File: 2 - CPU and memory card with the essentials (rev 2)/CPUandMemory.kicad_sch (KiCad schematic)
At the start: 9 parts, among them U10 AS6C4008, U7 Z84C0010, U8 SST39SF010, U9 AS6C4008

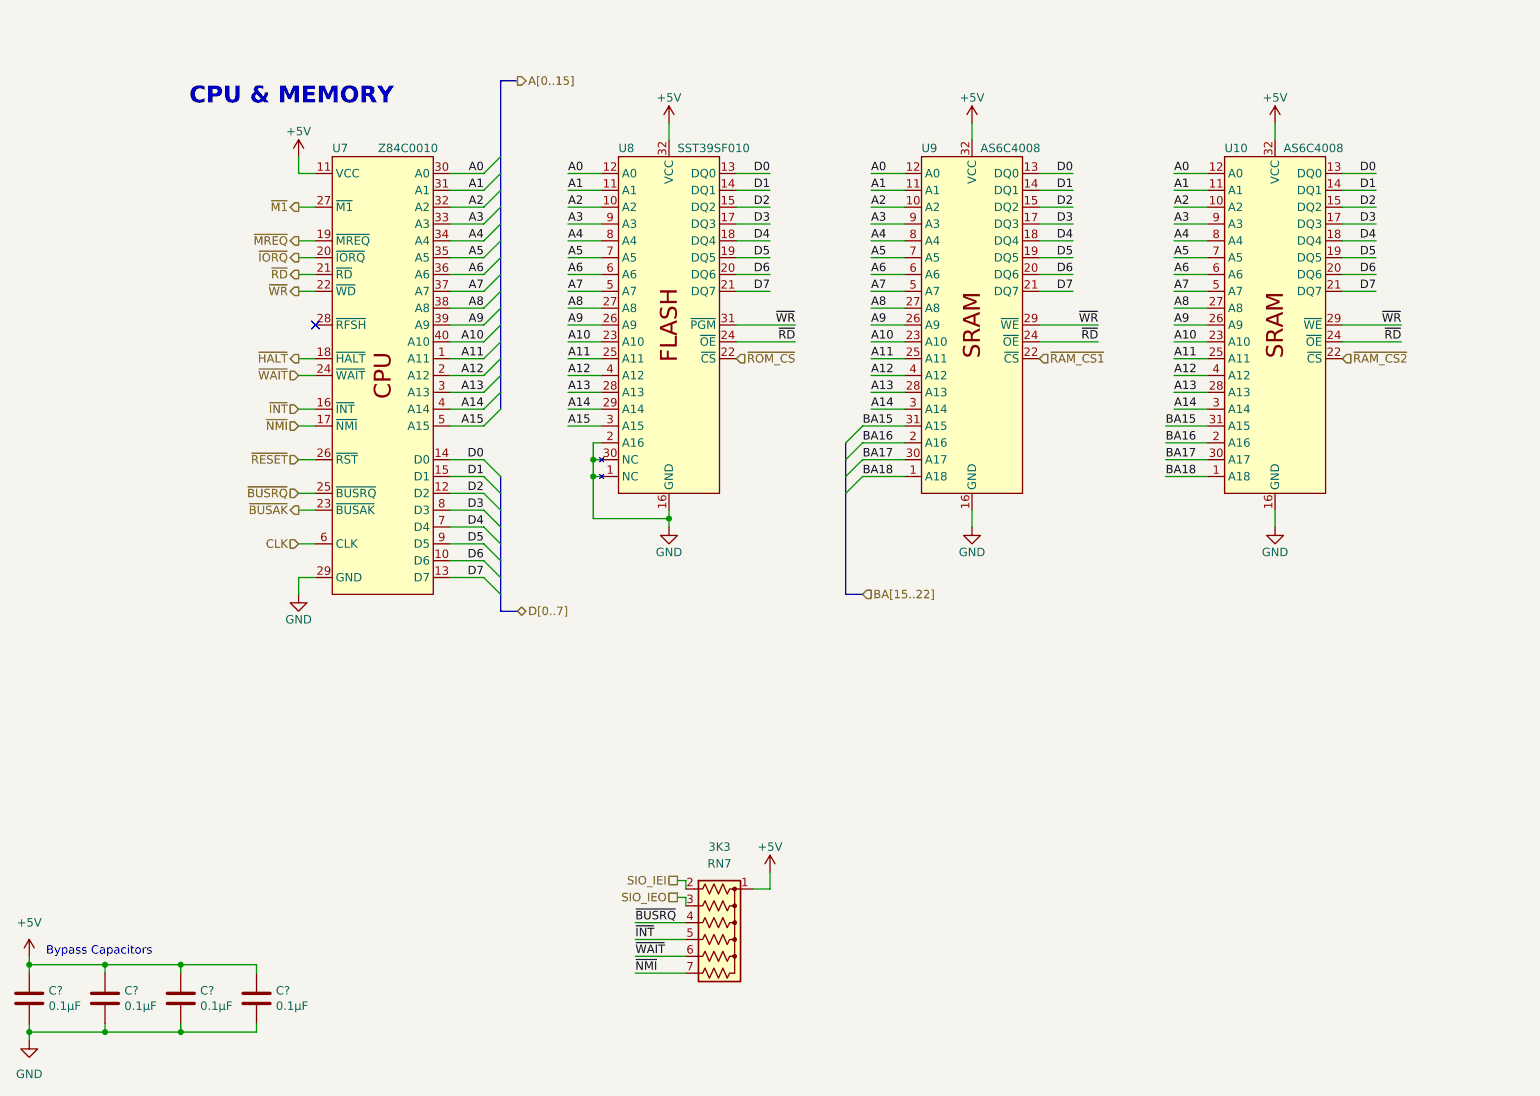
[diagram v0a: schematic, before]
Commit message: Trying to hash out the flaws
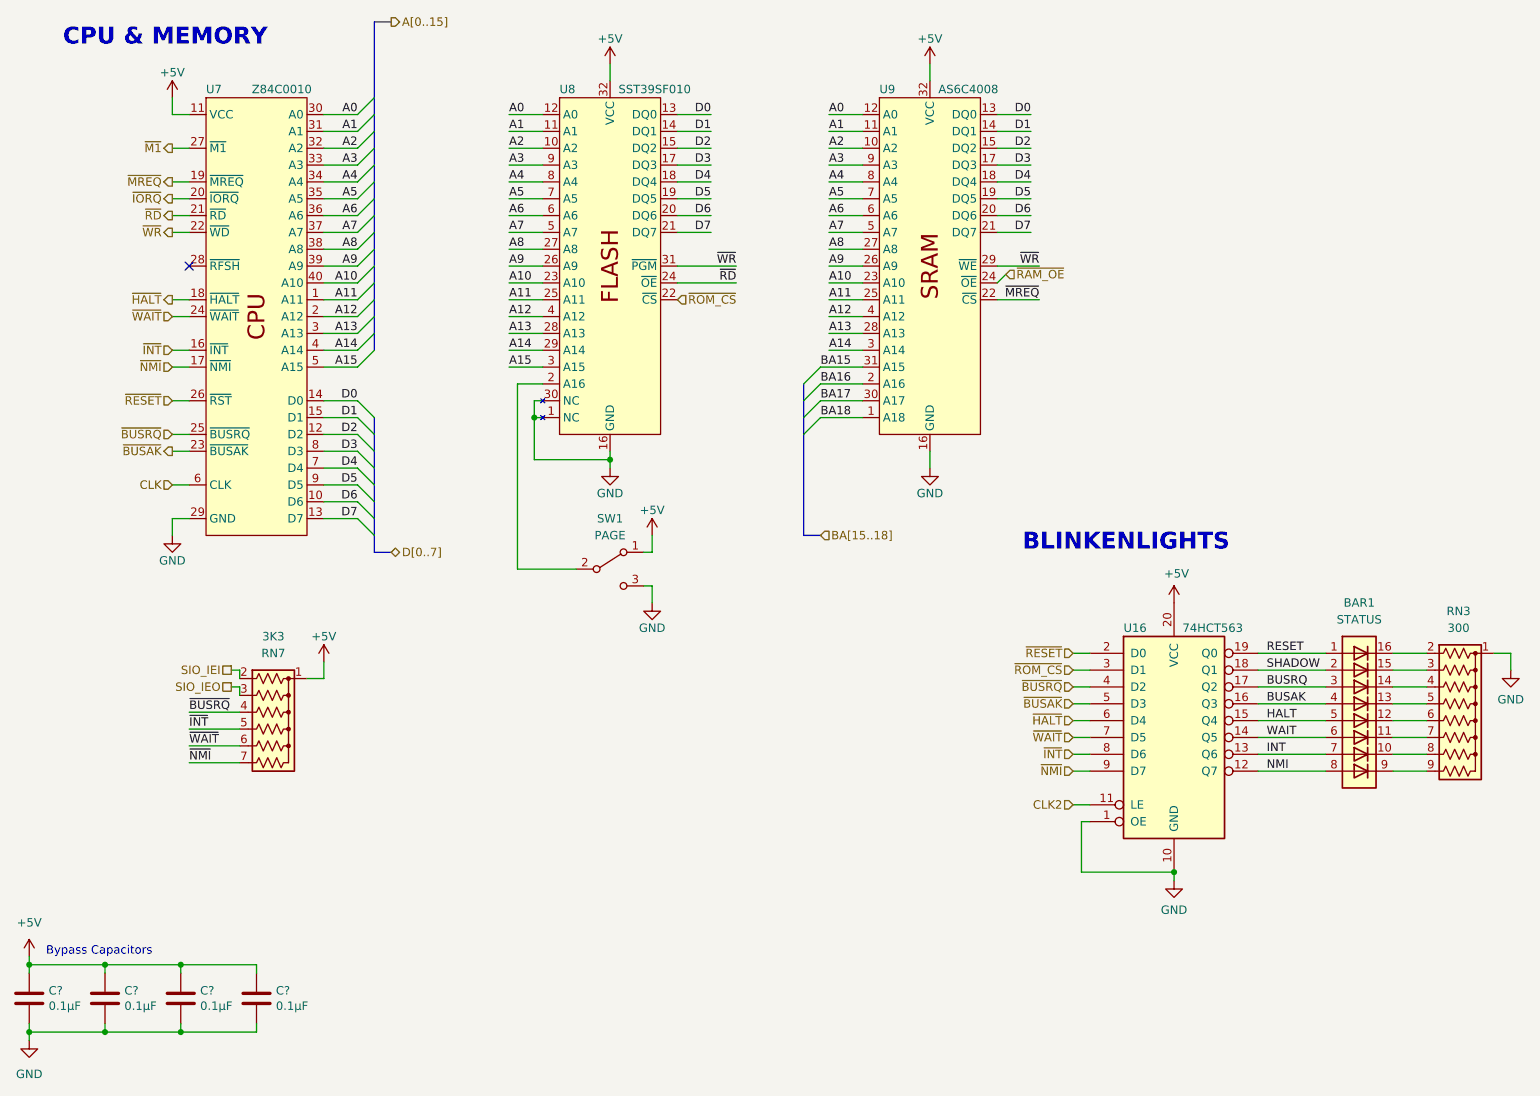
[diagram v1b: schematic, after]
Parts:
- removed C?: 0.1µF, Capacitor_THT:C_Disc_D3.0mm_W1.6mm_P2.50mm, symbol Device:C
- removed U10: AS6C4008, Package_DIP:DIP-32_W15.24mm_Socket, symbol 0_Library:AS6C4008
- added BAR1: STATUS, 0_Library:BAR_GRAPH_8, symbol 0_Library:BAR_GRAPH_8
- added C?: 0.1µF, Capacitor_THT:C_Disc_D3.0mm_W1.6mm_P2.50mm, symbol Device:C
- added RN3: 300, Resistor_THT:R_Array_SIP9, symbol Device:R_Network08_US
- added SW1: PAGE, 0_Library:Microswitch_2.54mm_spacing, symbol Switch:SW_SPDT
- added U16: 74HCT563, Package_DIP:DIP-20_W7.62mm_Socket, symbol 0_Library:74HC563
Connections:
- net ~{RAM_CS1} is gone; now on net ~{MREQ}: U9.22 (~{CS})
- net +5V: now also C?.1, SW1.1 (A), U16.20 (VCC)
- net GND: now also C?.2, RN3.1 (common), SW1.3 (C), U16.1 (OE), U16.10 (GND); no longer U8.2 (A16)
- net ~{BUSAK}: now also U16.5 (D3)
- net ~{BUSRQ}: now also U16.4 (D2)
- net ~{HALT}: now also U16.6 (D4)
- net ~{INT}: now also U16.8 (D6)
- net ~{NMI}: now also U16.9 (D7)
- net ~{RD}: no longer U9.24 (~{OE})
- net ~{RESET}: now also U16.2 (D0)
- net ~{ROM_CS}: now also U16.3 (D1)
- net ~{WAIT}: now also U16.7 (D5)
- new net: SW1.2 (B), U8.2 (A16)
- new net: BAR1.10 (A), RN3.8 (R7)
- new net: BAR1.11 (K), RN3.7 (R6)
- new net: BAR1.12 (K), RN3.6 (R5)
- new net: BAR1.13 (K), RN3.5 (R4)
- new net: BAR1.14 (K), RN3.4 (R3)
- new net: BAR1.15 (K), RN3.3 (R2)
- new net: BAR1.16 (K), RN3.2 (R1)
- new net: BAR1.9 (A), RN3.9 (R8)
- new net BUSAK: BAR1.4 (A), U16.16 (Q3)
- new net BUSRQ: BAR1.3 (A), U16.17 (Q2)
- new net CLK2: U16.11 (LE)
- new net HALT: BAR1.5 (A), U16.15 (Q4)
- new net INT: BAR1.7 (A), U16.13 (Q6)
- new net NMI: BAR1.8 (A), U16.12 (Q7)
- new net RESET: BAR1.1 (A), U16.19 (Q0)
- new net SHADOW: BAR1.2 (A), U16.18 (Q1)
- new net WAIT: BAR1.6 (A), U16.14 (Q5)
- new net ~{RAM_OE}: U9.24 (~{OE})
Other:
- note added: "BLINKENLIGHTS"
- moved on the sheet: RN7, U7, U8, U9
